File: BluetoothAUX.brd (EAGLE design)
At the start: 39.4 x 39.4 mm, 26 parts, among them IC1 NE5532D, X2 MINI-USB-SCHIELD-32005-201, X3 STEREOJACK

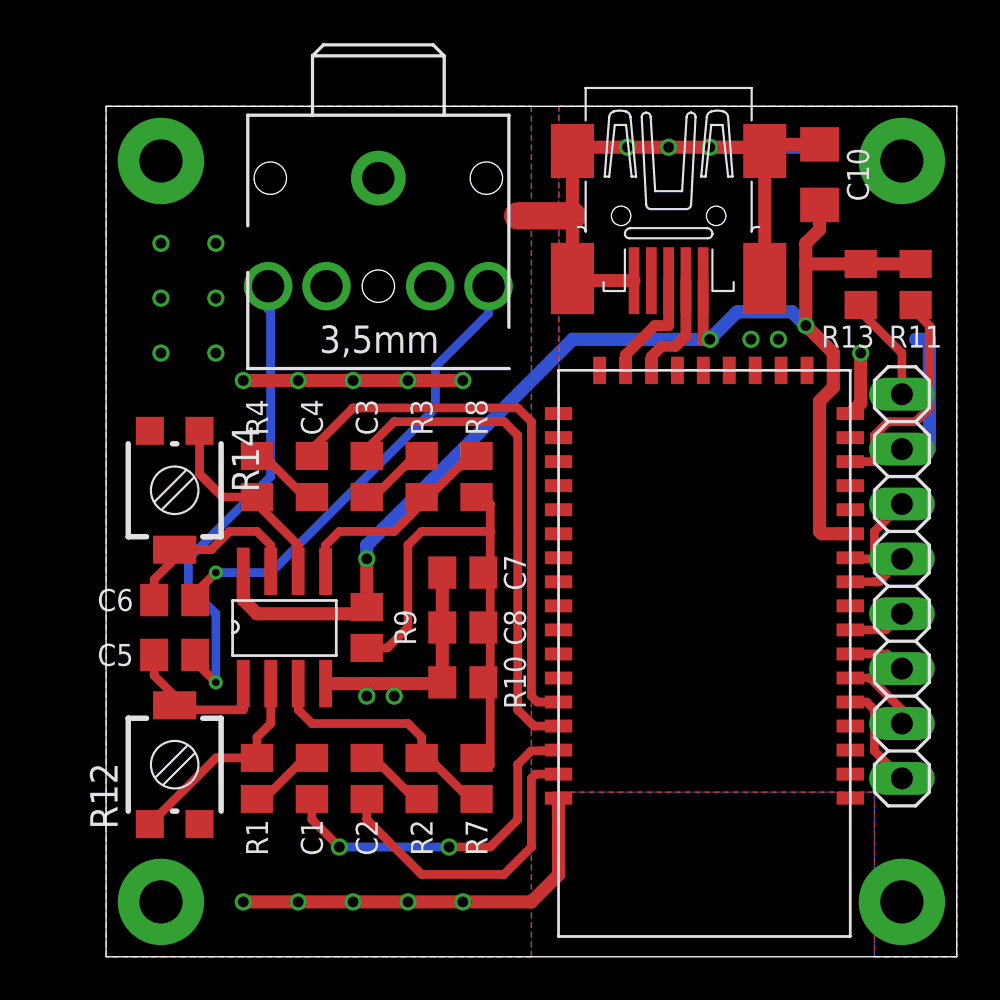
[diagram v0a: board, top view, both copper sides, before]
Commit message: TPA6132A
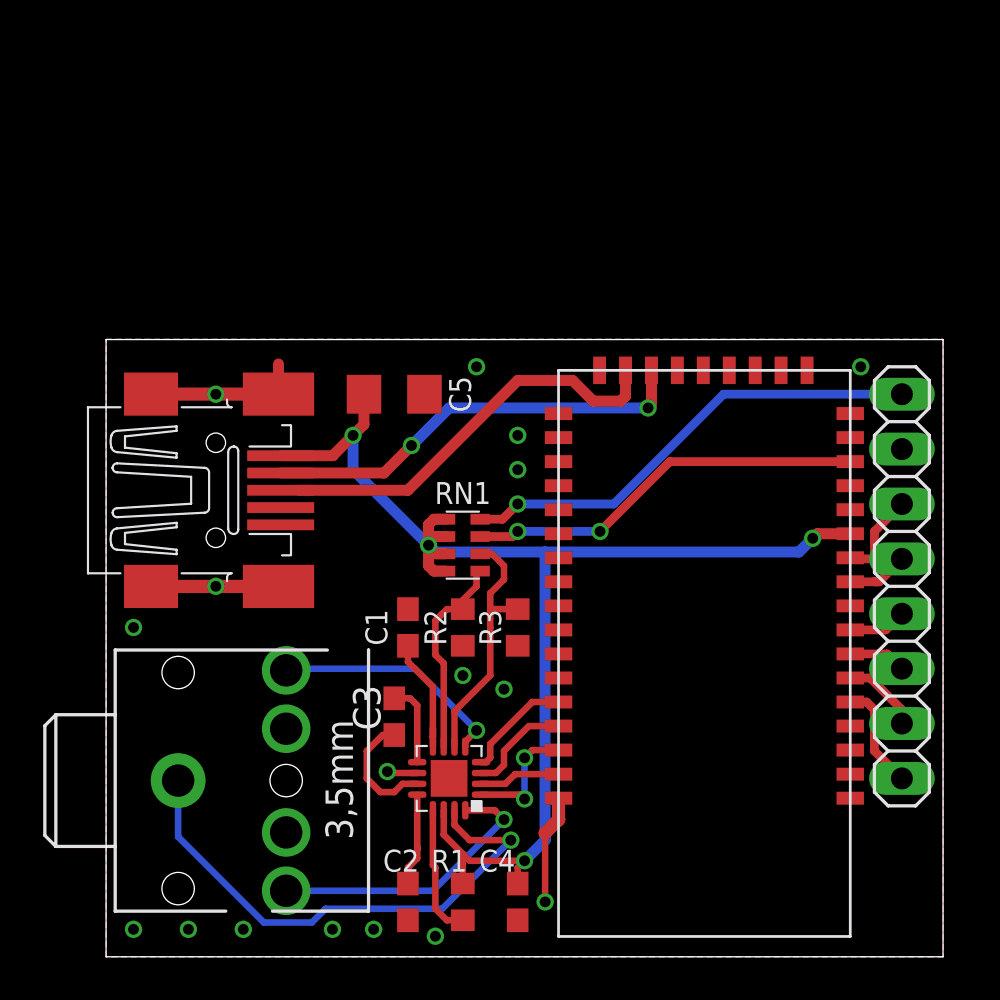
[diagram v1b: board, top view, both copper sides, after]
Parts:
- removed C10: 10uF, rcl:C1206
- removed C6: 1uF, rcl:C0805
- removed C7: 4.7uF, rcl:C0805
- removed C8: 10nF, rcl:C0805
- removed IC1: NE5532D, BT:SO08
- removed R10, R9: 100K, rcl:R0805
- removed R11, R13, R4, R7, R8: 10K, rcl:R0805
- removed R12, R14: (no value), resistor:RTRIM3314G
- removed X3: STEREOJACK, adafruit:STX3100
- added IC2: TPA6132A2, texas:QFN16
- added RN1: CTS742C083, resistor-net:CTS742C083
- added X1: STEREOJACK, adafruit:STX3100
- C1, C3: device rcl:C0805 -> resistor:C0603
- C2, C4: value 1uF -> 2.2uF; device rcl:C0805 -> resistor:C0603
- C5: value 1uF -> 10uF; device rcl:C0805 -> rcl:C1206
- R1: device rcl:R0805 -> resistor:R0603
- R2, R3: value 10K -> (none); device rcl:R0805 -> resistor:R0603
- moved X2 24.5 mm to (50.8, 36.8), turned to 0 degrees
- moved C4 21.9 mm to (64.8, 17.8)
- moved C5 15.8 mm to (59.1, 41.3)
- moved C3 11.2 mm to (59.1, 26.4), turned to 90 degrees
- moved R1 11.1 mm to (62.2, 17.8)
- moved C1 8.28 mm to (59.7, 30.5)
- moved R3 8.28 mm to (64.8, 30.5), turned to 90 degrees
- moved R2 7.24 mm to (62.2, 30.5)
- moved C2 6.02 mm to (59.7, 17.8), turned to 270 degrees
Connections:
- removed net N$1: IC1.2, R1.2, R12.3
- removed net N$10: C6.1, IC1.7, R14.2
- removed net N$11: C7.1, C8.1, R10.2, R7.1, R8.2, R9.1
- removed net N$2: IC1.3, R2.2, R7.2
- removed net N$3: IC1.6, R14.3, R4.2
- removed net N$4: IC1.5, R3.2, R8.1
- removed net N$5: C1.2, R1.1
- removed net N$6: C2.2, R2.1
- removed net N$7: C3.2, R3.1
- removed net N$8: C4.2, R4.1
- removed net N$9: C5.1, IC1.1, R12.2
- removed net SPK_L: C5.2, X3.5
- removed net SPK_R: C6.2, X3.2
- new net N$14: IC2.5, X1.2
- new net N$20: IC2.16, X1.5
- new net N$26: C3.1, IC2.11
- new net N$27: C3.2, IC2.9
- new net N$28: C1.1, IC2.8
- new net N$29: C2.1, IC2.12
- new net N$30: IC2.13, R1.1
- new net N$31: IC2.6, R3.2, RN1.6
- new net N$32: IC2.7, R2.2, RN1.5
- new net SGND: IC2.15, X1.1
- net +5V: now also C4.1, C5.1, IC2.14, R1.2, RN1.1, RN1.2, RN1.3, RN1.4; no longer C10.1, IC1.8, R11.1, R13.2, R9.2
- net COM: now also RN1.8; no longer R13.1
- net GND: now also C1.2, C2.2, C4.2, C5.2, IC2.10, R2.1, R3.1; no longer C10.2, C7.2, C8.2, IC1.4, R10.1, X3.1
- net N$13: now also RN1.7; no longer R11.2
- net SPK_LN: now also IC2.1; no longer C1.1
- net SPK_LP: now also IC2.2; no longer C2.1
- net SPK_RN: now also IC2.4; no longer C4.1
- net SPK_RP: now also IC2.3; no longer C3.1
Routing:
- net GND: track 84.2 -> 19.9 mm, vias 24 -> 17
- net SGND: track 0.00 -> 24.8 mm, vias 0 -> 1
- net N$11: track 24.7 -> 0.00 mm
- net SPK_L: track 22.2 -> 0.00 mm, vias 1 -> 0
- net SPK_R: track 21.6 -> 0.00 mm, vias 1 -> 0
- net SPK_RN: track 25.6 -> 5.12 mm
- net SPK_RP: track 23.0 -> 4.87 mm
- net COM: track 4.92 -> 21.9 mm, vias 0 -> 1
- net N$18: track 5.18 -> 20.1 mm, vias 0 -> 2
- net N$19: track 5.35 -> 20.2 mm
- net N$20: track 0.00 -> 13.4 mm, vias 0 -> 1
- net N$31: track 0.00 -> 11.9 mm
- net N$2: track 11.7 -> 0.00 mm
- net N$14: track 0.00 -> 11.0 mm, vias 0 -> 1
- net SPK_LP: track 14.7 -> 3.78 mm
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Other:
- board size 39.4 x 39.4 mm -> 38.7 x 28.6 mm
